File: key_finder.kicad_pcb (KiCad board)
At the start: 2 copper layers, 45.7 x 52.1 mm, 27 parts, among them J1 Conn_ARM_JTAG_SWD_10, SW1 SW_Push, SW2 SW_Push, U1 NRF52832, X1 32MHz, X2 32.768kHz

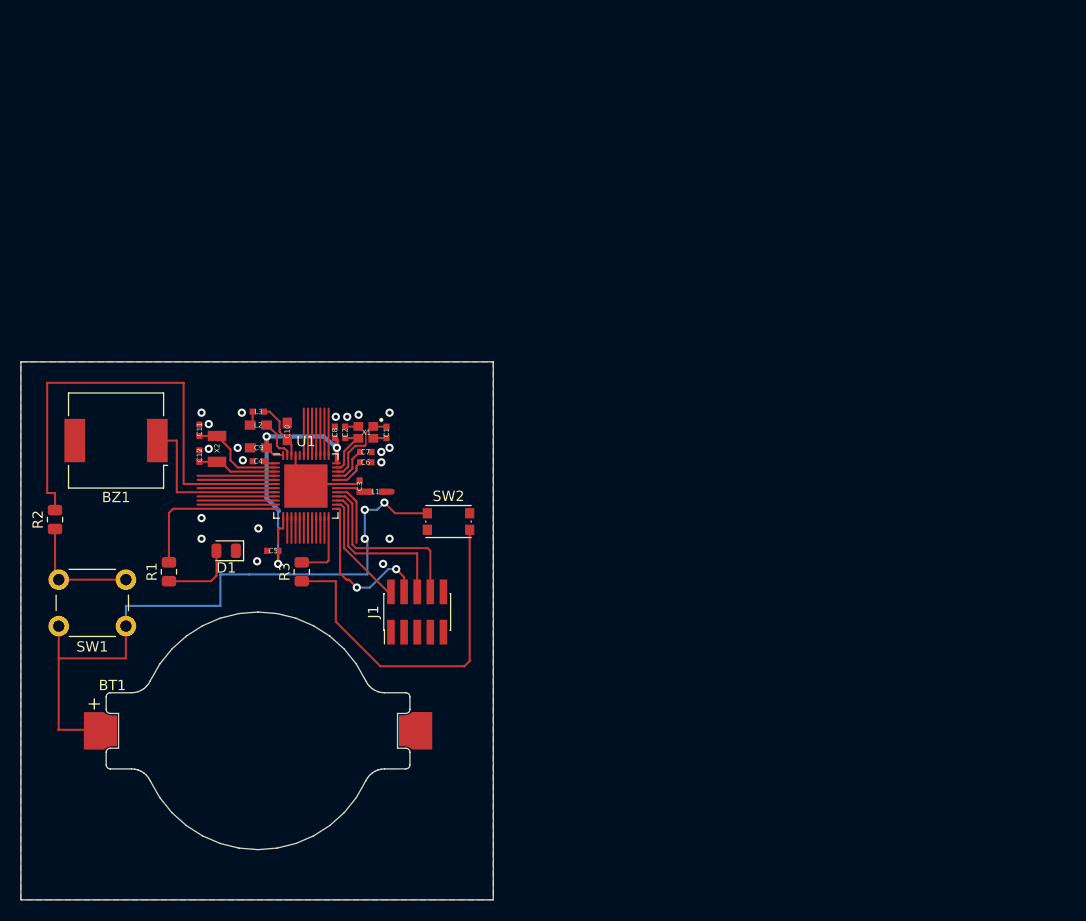
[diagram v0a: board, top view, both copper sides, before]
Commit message: sceance 2
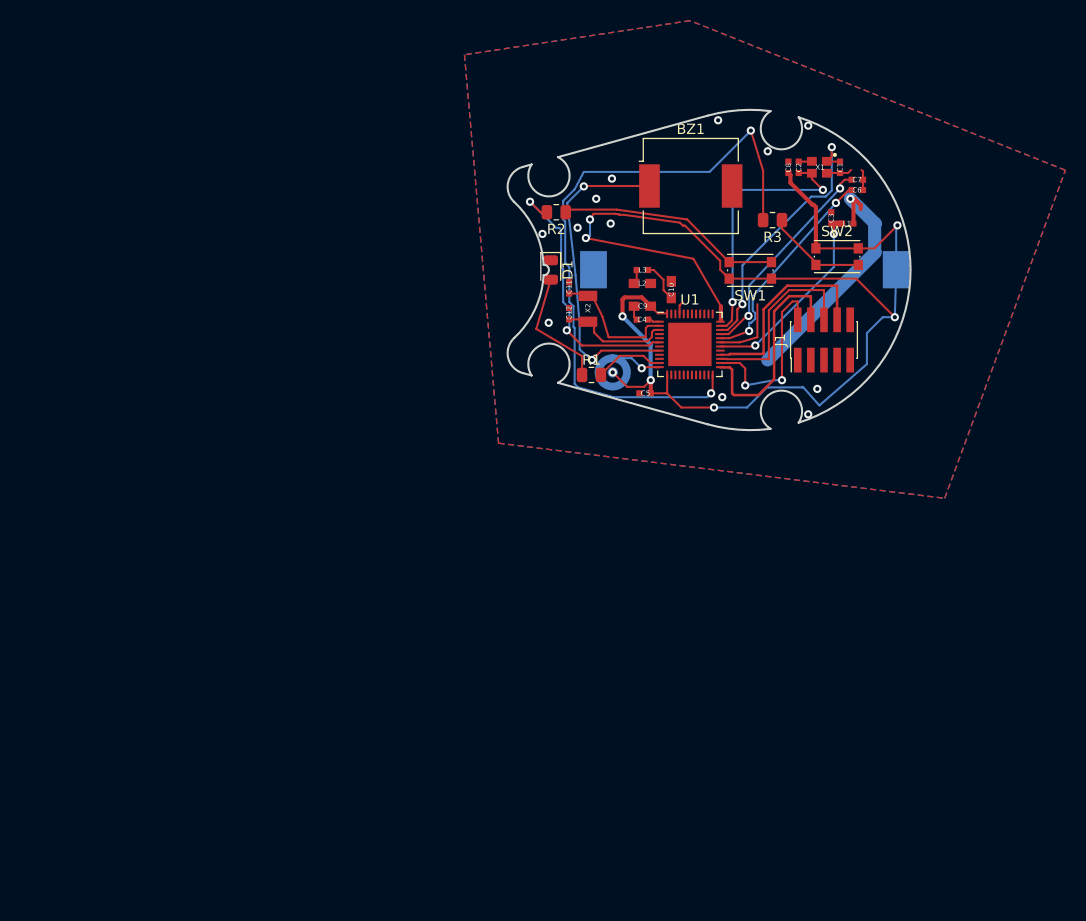
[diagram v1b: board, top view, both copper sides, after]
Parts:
- added MK1: Microphone, Sensor_Audio:CUI_CMC-4013-SMT, B.Cu at (179.2, 95.0)
- BT1: footprint Battery:BatteryHolder_Keystone_1057_1x2032 -> Battery:BatteryHolder_Keystone_1060_1x2032; moved to B.Cu
- SW1: footprint Button_Switch_THT:SW_PUSH_6mm_H7.3mm -> Button_Switch_SMD:SW_Push_1P1T_NO_CK_KMR2
- moved SW1 69.6 mm to (192.5, 85.1)
- moved BT1 64.9 mm to (192.0, 85.1), turned to 180 degrees
- moved BZ1 60.8 mm to (186.8, 77.0), turned to 0 degrees
- moved R2 56.9 mm to (173.7, 79.5), turned to 180 degrees
- moved R3 56.9 mm to (194.7, 80.3), turned to 180 degrees
- moved C6 54.4 mm to (202.9, 77.4)
- moved C7 54.4 mm to (202.9, 76.4)
- moved C3 52.5 mm to (200.3, 80.0)
- moved L1 52.5 mm to (201.9, 80.6)
- moved C1 50.8 mm to (201.2, 75.2)
- moved C2 50.8 mm to (197.2, 75.2)
- moved C8 50.8 mm to (196.2, 75.2)
- moved X1 50.8 mm to (199.2, 75.2)
- moved J1 47.4 mm to (199.6, 91.9)
- moved SW2 45.5 mm to (200.9, 83.8)
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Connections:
- net /P0.00/XL1 renamed Net-(U1-P0.00/XL1@02)
- net /P0.01/XL2 renamed Net-(U1-P0.01/XL2@03)
- C1 pad 1: X1 -> Net-(U1-XC1@34)
- C2 pad 1: N$3 -> Net-(U1-XC2@35)
- C3 pad 1: ANT -> Net-(U1-ANT@30)
- C5 pad 1: VDD_P3V3 -> VCC
- C6 pad 1: DEC2 -> /DEC2
- C7 pad 1: DEC3 -> /DEC3
- C8 pad 1: VDD_P3V3 -> VCC
- C9 pad 1: VDD_P3V3 -> VCC
- L1 pad 1: ANT -> Net-(U1-ANT@30)
- R1 pad 2: /P0.10 -> /P0.09
- X1 pad 1: X1 -> Net-(U1-XC1@34)
- X1 pad 3: N$3 -> Net-(U1-XC2@35)
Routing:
- net VCC: track 68.3 -> 132.5 mm, vias 3 -> 8
- net /P0.21/RESET: track 6.89 -> 63.8 mm, vias 0 -> 2
- net VDD_P3V3: track 26.9 -> 0.00 mm, vias 3 -> 0
- net Net-(U1-XC1@34): track 0.00 -> 26.2 mm, vias 0 -> 2
- net Net-(U1-XC2@35): track 0.00 -> 25.7 mm, vias 0 -> 2
- net Net-(R3-Pad1): track 34.9 -> 9.80 mm
- net RF: track 0.95 -> 25.1 mm, vias 0 -> 1
- net /DEC3: track 0.00 -> 21.2 mm, vias 0 -> 2
- net /DEC2: track 0.00 -> 20.9 mm, vias 0 -> 2
- net Net-(U1-ANT@30): track 0.00 -> 19.6 mm, vias 0 -> 2
- net /P0.04: track 44.9 -> 26.0 mm, vias 0 -> 2
- net /P0.06: track 16.4 -> 31.4 mm, vias 0 -> 2
- net GND: track 27.1 -> 15.2 mm, vias 19 -> 12
- net Net-(R2-Pad1): track 11.6 -> 21.5 mm
- net /P0.10: track 15.2 -> 5.42 mm, vias 0 -> 1
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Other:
- board size 45.7 x 52.1 mm -> 39 x 31 mm
